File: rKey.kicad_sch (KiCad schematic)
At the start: 41 parts, among them IC1 BDX34C, J1 Conn_01x06, K1 RT42xxxx, Q1 BC337, Q2 BC337, Q3 BC337, Q4 BC337, Q5 BC327, Q8 BC337, U1 TL084BCN, U2 LM7810_TO220

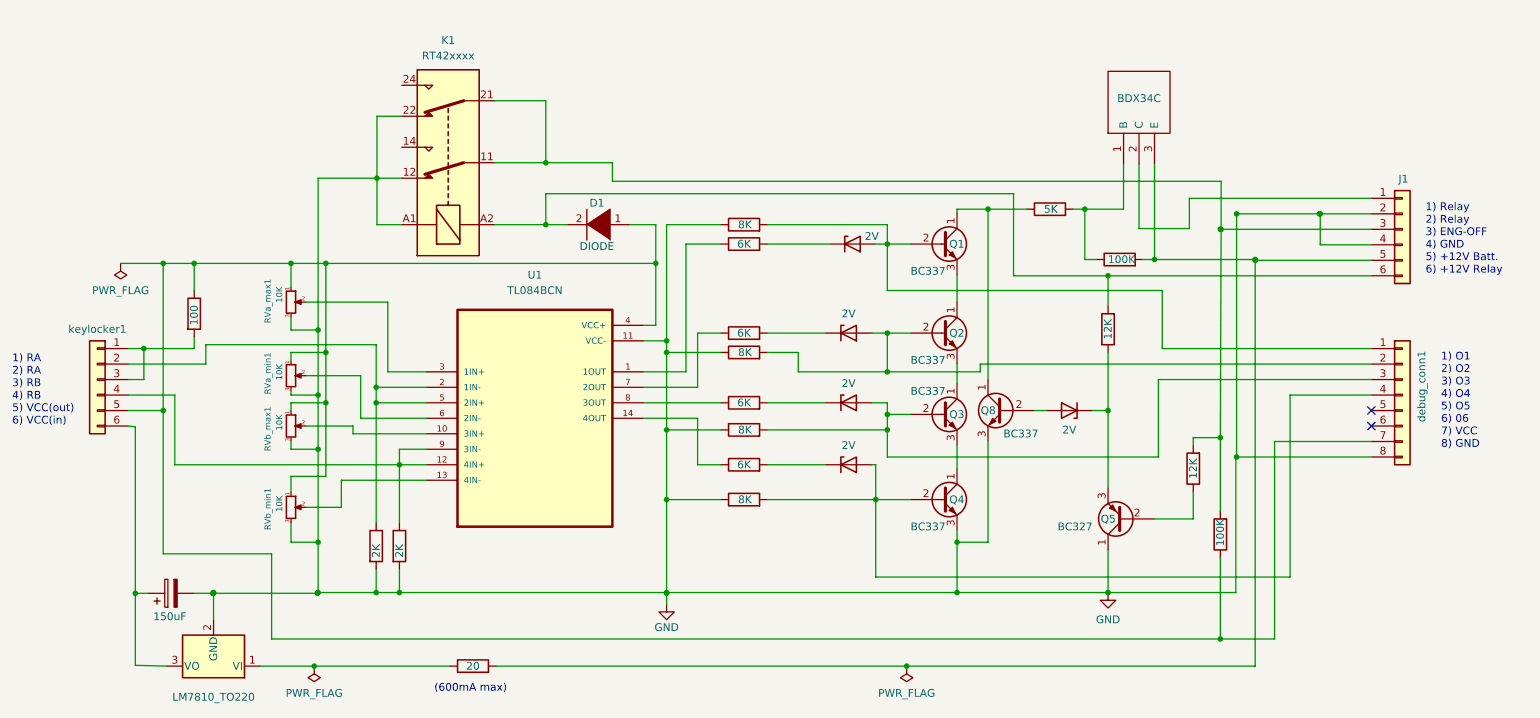
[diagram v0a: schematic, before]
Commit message: fixes
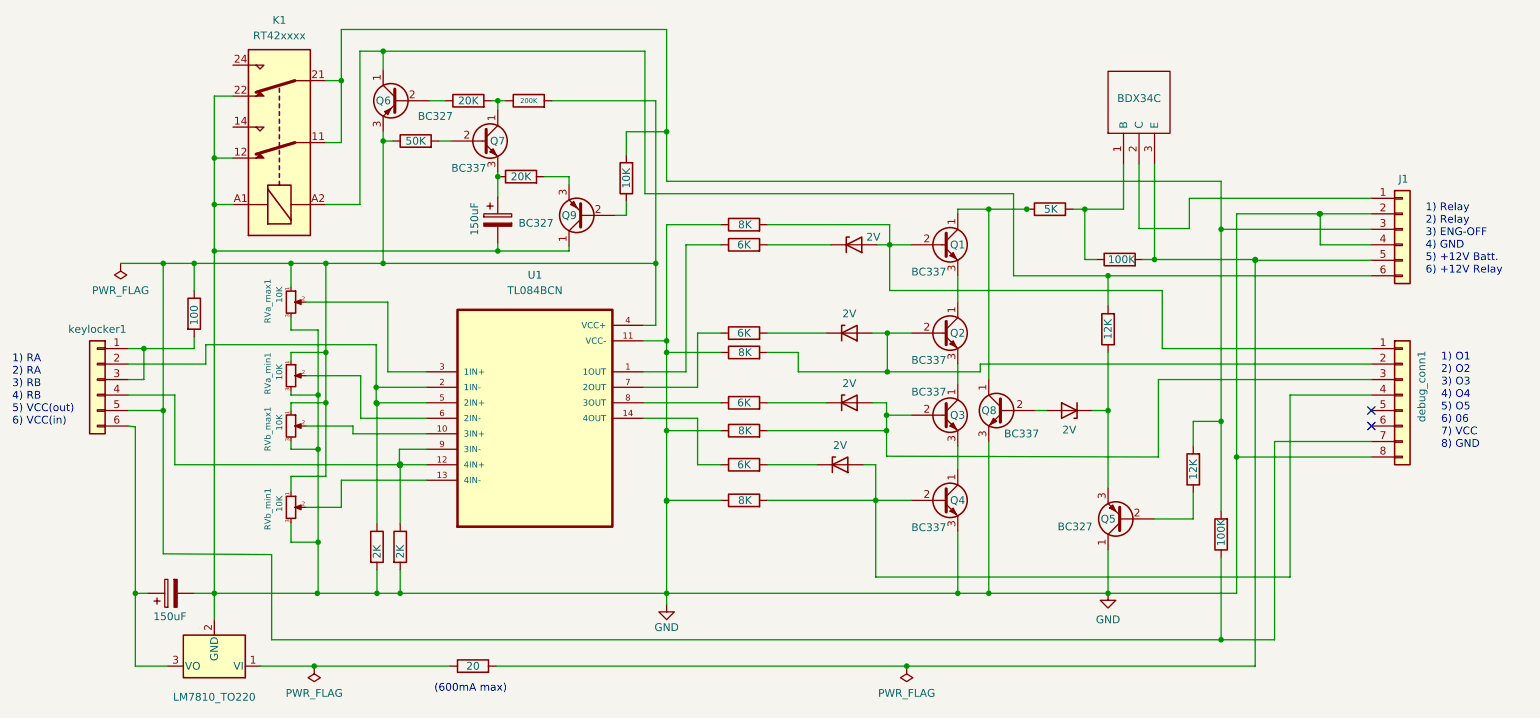
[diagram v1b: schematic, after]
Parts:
- removed D1: DIODE, Diode_THT:D_DO-34_SOD68_P7.62mm_Horizontal, symbol pspice:DIODE
- added C2: 150uF, Capacitor_THT:CP_Radial_D7.5mm_P2.50mm, symbol Device:C_Polarized
- added Q6, Q9: BC327, Package_TO_SOT_THT:TO-92L_Inline_Wide, symbol Transistor_BJT:BC327
- added Q7: BC337, Package_TO_SOT_THT:TO-92L_Inline_Wide, symbol Transistor_BJT:BC337
- added R18: 50K, Resistor_THT:R_Axial_DIN0204_L3.6mm_D1.6mm_P5.08mm_Horizontal, symbol Device:R
- added R19, R20: 20K, Resistor_THT:R_Axial_DIN0204_L3.6mm_D1.6mm_P5.08mm_Horizontal, symbol Device:R
- added R21: 200K, Resistor_THT:R_Axial_DIN0204_L3.6mm_D1.6mm_P5.08mm_Horizontal, symbol Device:R
- added R22: 10K, Resistor_THT:R_Axial_DIN0204_L3.6mm_D1.6mm_P5.08mm_Horizontal, symbol Device:R
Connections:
- net GND: now also C2.2, Q9.1 (C)
- net at J1.3 (Pin_3), K1.11, K1.21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: now also R22.2
- net at R1.1, R14.1, RVa_max1.1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: now also Q6.3 (E), R18.1, R21.2
- net at J1.6 (Pin_6), K1.A2, R9.2: now also Q6.1 (C)
- new net: Q9.2 (B), R22.1
- new net: Q7.2 (B), R18.2
- new net: C2.1, Q7.3 (E), R20.1
- new net: Q9.3 (E), R20.2
- new net: Q6.2 (B), R19.1
- new net: Q7.1 (C), R19.2, R21.1
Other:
- moved on the sheet: K1
